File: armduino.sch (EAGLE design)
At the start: 61 parts, among them IC1 78D2, IC3 LM1117-3.3V, Q1 12MHz, Q2 12MHz, T1 BC857, T2 BC857, U1 LPC11U35FBD48/401, U2 MKE02Z64VLD4, X1 POWERSUPPLY_DC21MMX, X2 USB-B_TH

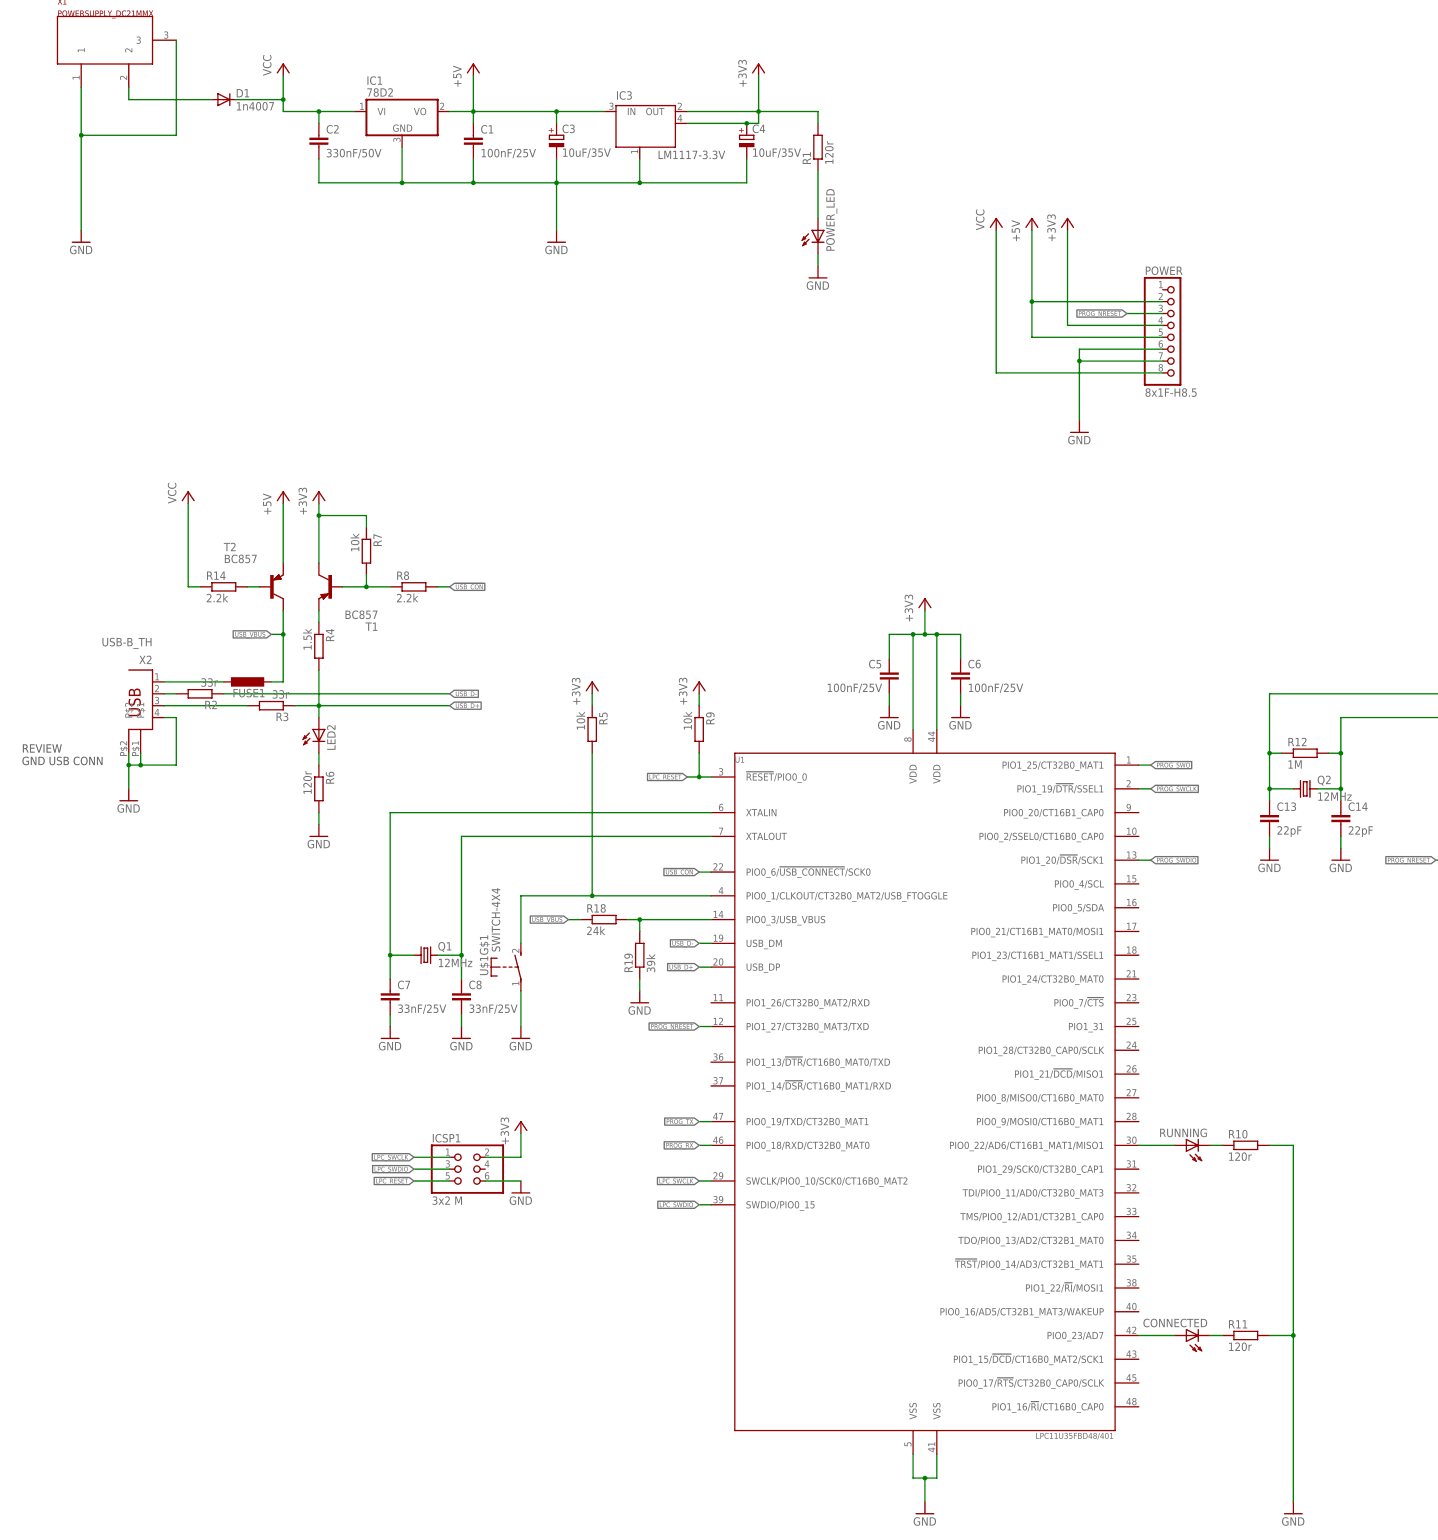
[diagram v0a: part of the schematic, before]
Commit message: Version 0.4
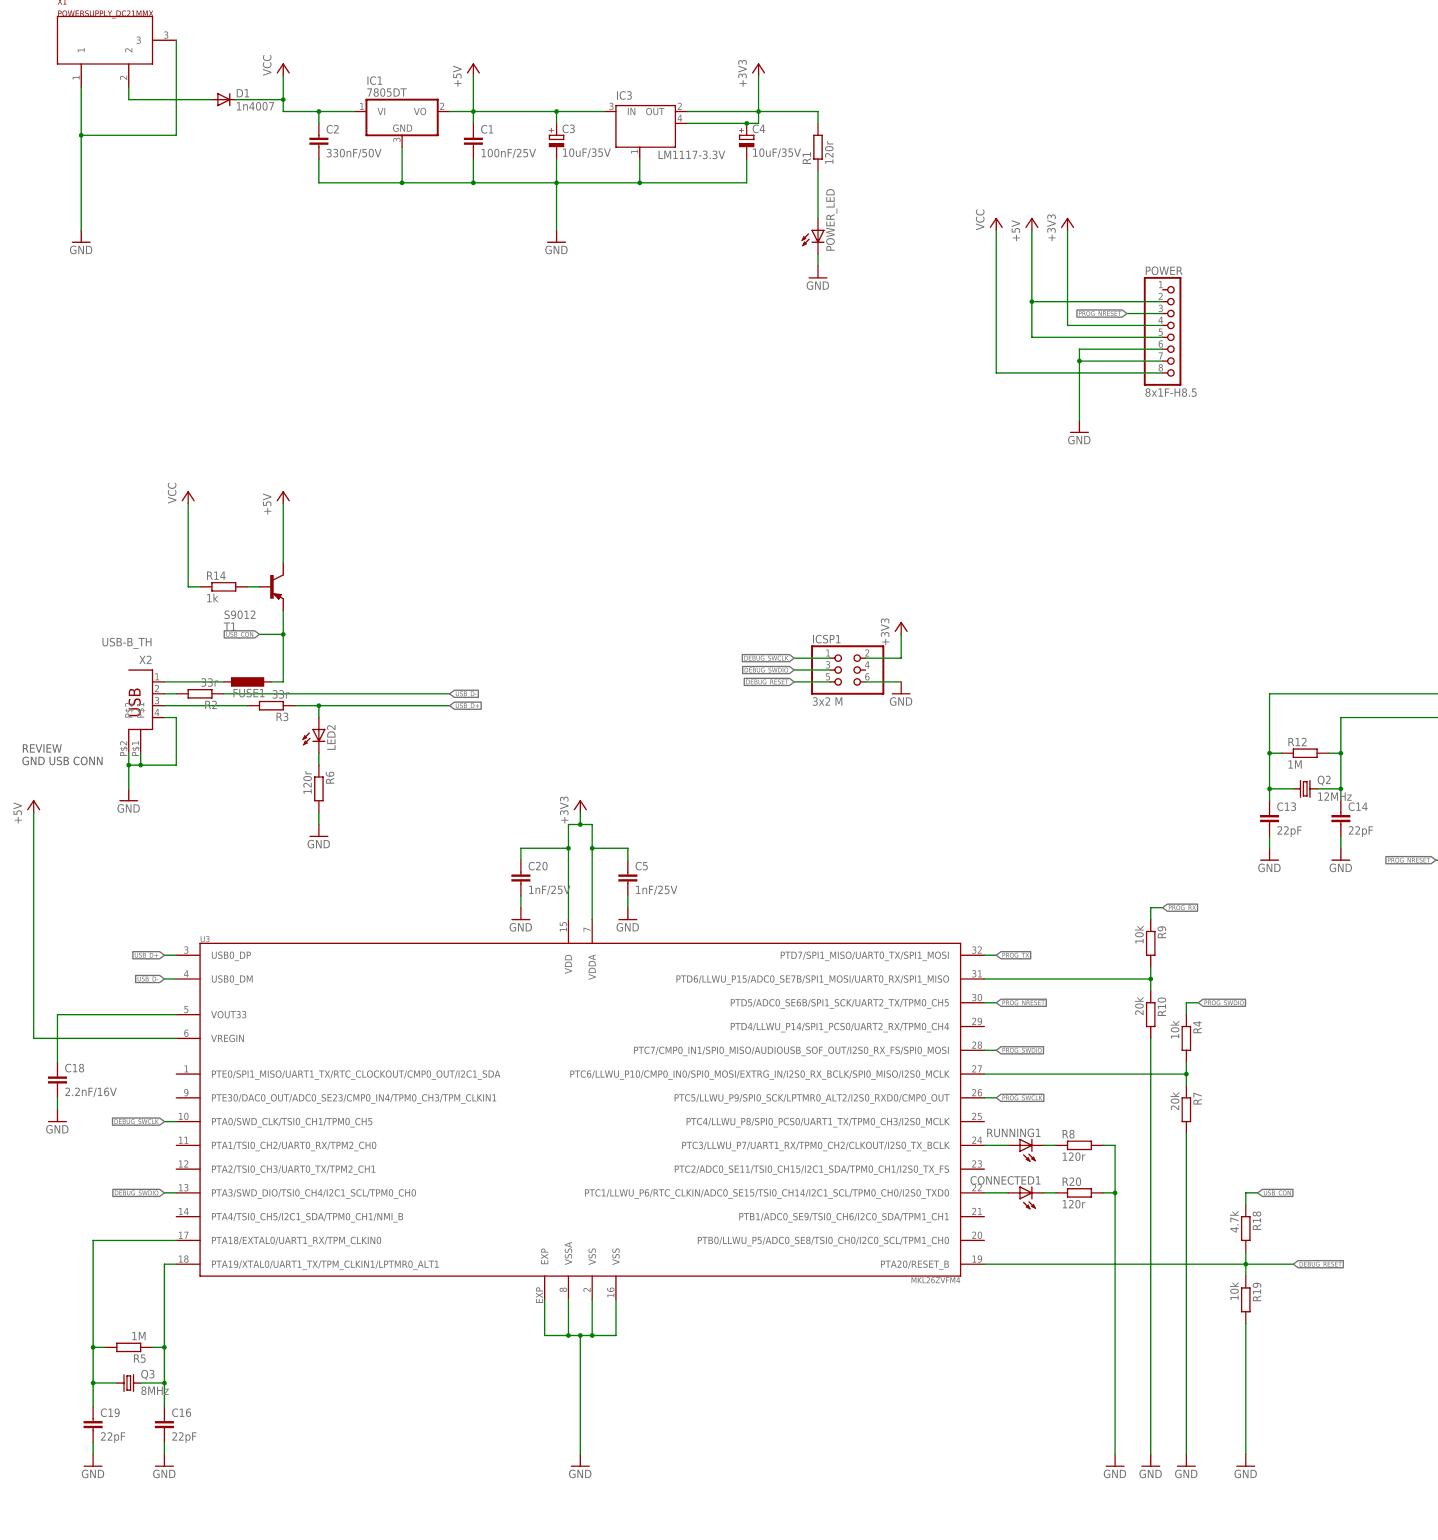
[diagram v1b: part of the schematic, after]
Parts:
- removed C6: 100nF/25V, rcl:C-EUC0805K
- removed C7, C8: 33nF/25V, rcl:C-EUC0805K
- removed CONNECTED, RUNNING: (no value), led:LEDCHIP-LED0805
- removed Q1: 12MHz, crystal:CRYSTALSM49
- removed R11: 120r, rcl:R-EU_M0805
- removed T2: BC857, transistor:BC857A-PNP-SOT23-BEC
- removed U$1: SWITCH-4X4, pessoal:SWITCH-4X4
- removed U1: LPC11U35FBD48/401, NXP_By_element14_Batch_1:LPC11U35FBD48/401
- added C16, C19: 22pF, rcl:C-EUC0603K
- added C18: 2.2nF/16V, rcl:C-EUC0805K
- added C20: 1nF/25V, rcl:C-EUC0805K
- added CONNECTED1, RUNNING1: (no value), led:LEDCHIP-LED0805
- added Q3: 8MHz, crystal:CRYSTALHC49S
- added R20: 120r, rcl:R-EU_M0805
- added U3: MKL26ZVFM4, freescale:MKL26ZVFM4
- C5: value 100nF/25V -> 1nF/25V
- IC1: value 78D2 -> 7805DT; device linear:78D2 -> linear:7805DT
- R10: value 120r -> 20k
- R14: value 2.2k -> 1k
- R18: value 24k -> 4.7k
- R19: value 39k -> 10k
- R4: value 1.5k -> 10k
- R5: value 10k -> 1M
- R7: value 10k -> 20k
- R8: value 2.2k -> 120r
- T1: value BC857 -> S9012; device transistor:BC857A-PNP-SOT23-BEC -> transistor:-PNP-SOT23-BCE
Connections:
- removed net !USB_CON: R8.2, U1.PIO0_6/!USB_CONNECT!/SCK0
- removed net LPC_RESET: ICSP1.5, R9.2, U1.!RESET!/PIO0_0
- removed net LPC_SWCLK: ICSP1.1, U1.SWCLK/PIO0_10/SCK0/CT16B0_MAT2
- removed net LPC_SWDIO: ICSP1.3, U1.SWDIO/PIO0_15
- removed net N$10: C8.1, Q1.2, U1.XTALOUT
- removed net N$15: R10.1, RUNNING.C
- removed net N$16: CONNECTED.C, R11.1
- removed net N$9: C7.1, Q1.1, U1.XTALIN
- removed net PROG_SWO: U1.PIO1_25/CT32B0_MAT1
- removed net USB_VBUS: FUSE1.2, R18.1, T2.C
- new net DEBUG_RESET: ICSP1.5, R18.2, R19.1, U3.PTA20/RESET_B
- new net DEBUG_SWCLK: ICSP1.1, U3.PTA0/SWD_CLK/TSI0_CH1/TPM0_CH5
- new net DEBUG_SWDIO: ICSP1.3, U3.PTA3/SWD_DIO/TSI0_CH4/I2C1_SCL/TPM0_CH0
- new net N$12: CONNECTED1.C, R20.1
- new net N$25: C16.1, Q3.2, R5.1, U3.PTA19/XTAL0/UART1_TX/TPM_CLKIN1/LPTMR0_ALT1
- new net N$31: C18.1, U3.VOUT33
- new net USB_CON: FUSE1.2, R18.1, T1.E
- net +3V3: now also C20.1, U3.VDD, U3.VDDA; no longer C6.1, R5.1, R7.1, R9.1, T1.C, U1.VDD, U1.VDD@1
- net +5V: now also T1.C, U3.VREGIN; no longer T2.E
- net GND: now also C16.2, C18.2, C19.2, C20.2, R19.2, R20.2, R7.2, R8.2, U3.EXP, U3.VSS, U3.VSS@1, U3.VSSA; no longer C6.2, C7.2, C8.2, R11.2, R19.1, U$1G$1.P, U1.VSS, U1.VSS@1
- net N$11: now also RUNNING1.C; no longer R7.2, T1.B
- net N$13: now also RUNNING1.A, U3.PTC3/LLWU_P7/UART1_RX/TPM0_CH2/CLKOUT/I2S0_TX_BCLK; no longer RUNNING.A, U1.PIO0_22/AD6/CT16B1_MAT1/MISO1
- net N$14: now also CONNECTED1.A, U3.PTC1/LLWU_P6/RTC_CLKIN/ADC0_SE15/TSI0_CH14/I2C1_SCL/TPM0_CH0/I2S0_TXD0; no longer CONNECTED.A, U1.PIO0_23/AD7
- net N$22: now also T1.B; no longer T2.B
- net N$24: now also C19.1, Q3.1, R5.2, U3.PTA18/EXTAL0/UART1_RX/TPM_CLKIN0; no longer R18.2, R19.2, U1.PIO0_3/USB_VBUS
- net N$6: now also R10.1, R9.2, U3.PTD6/LLWU_P15/ADC0_SE7B/SPI1_MOSI/UART0_RX/SPI1_MISO; no longer R5.2, U$1G$1.S, U1.PIO0_1/CLKOUT/CT32B0_MAT2/USB_FTOGGLE
- net N$8: now also R4.2, R7.1, U3.PTC6/LLWU_P10/CMP0_IN0/SPI0_MOSI/EXTRG_IN/I2S0_RX_BCLK/SPI0_MISO/I2S0_MCLK; no longer R4.1, T1.E
- net PROG_NRESET: now also U3.PTD5/ADC0_SE6B/SPI1_SCK/UART2_TX/TPM0_CH5; no longer U1.PIO1_27/CT32B0_MAT3/TXD
- net PROG_RX: now also R9.1; no longer U1.PIO0_18/RXD/CT32B0_MAT0
- net PROG_SWCLK: now also U3.PTC5/LLWU_P9/SPI0_SCK/LPTMR0_ALT2/I2S0_RXD0/CMP0_OUT; no longer U1.PIO1_19/!DTR!/SSEL1
- net PROG_SWDIO: now also R4.1, U3.PTC7/CMP0_IN1/SPI0_MISO/AUDIOUSB_SOF_OUT/I2S0_RX_FS/SPI0_MOSI; no longer U1.PIO1_20/!DSR!/SCK1
- net PROG_TX: now also U3.PTD7/SPI1_MISO/UART0_TX/SPI1_MOSI; no longer U1.PIO0_19/TXD/CT32B0_MAT1
- net USB_D+: now also U3.USB0_DP; no longer R4.2, U1.USB_DP
- net USB_D-: now also U3.USB0_DM; no longer U1.USB_DM
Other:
- moved on the sheet: C5, ICSP1, R10, R18, R19, R4, R5, R7, R8, R9, T1
